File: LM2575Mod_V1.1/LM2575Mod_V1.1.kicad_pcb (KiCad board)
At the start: 2 copper layers, 99.1 x 63.5 mm, 24 parts, among them IC1 LM 2575 T-ADJ, X1 MKDSN1,5_2-5,08, X2 Val**, X3 MKDSN1,5_2-5,08

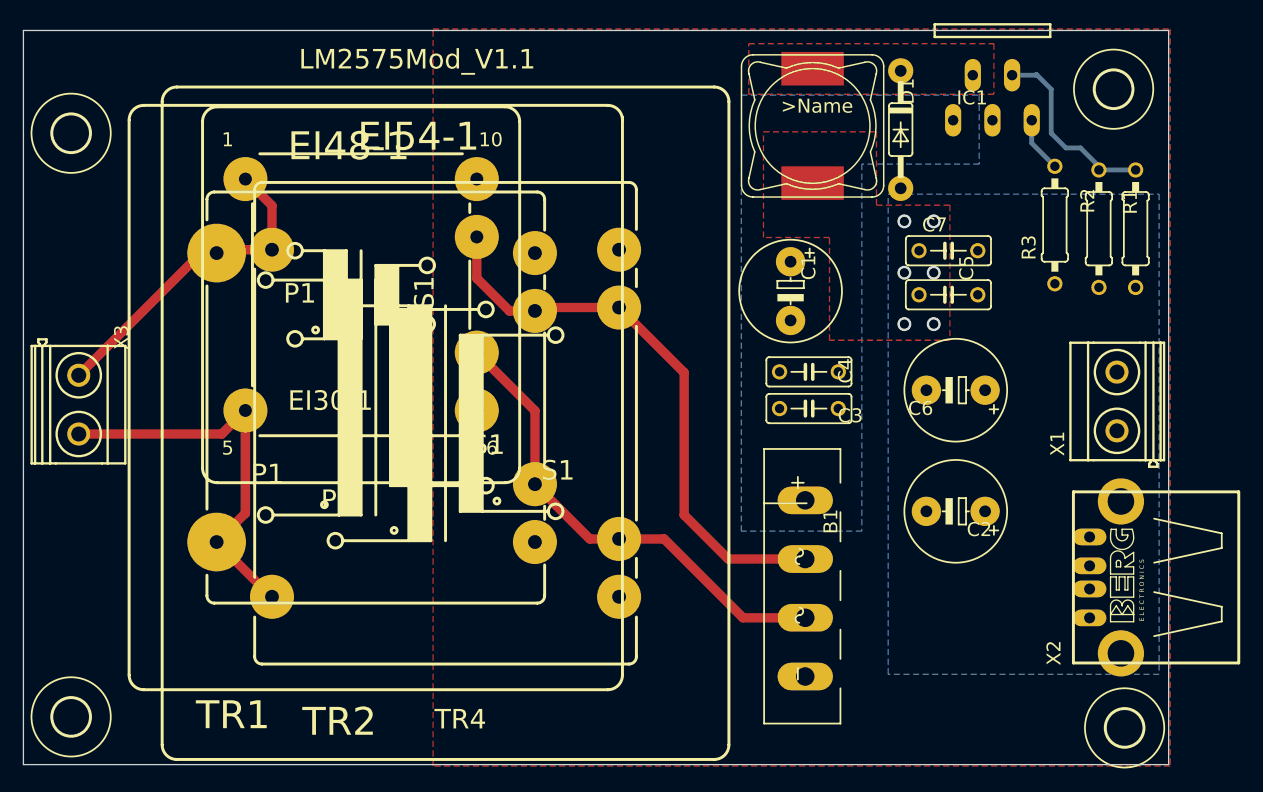
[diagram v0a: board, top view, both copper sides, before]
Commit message: lm2575_pwr V6
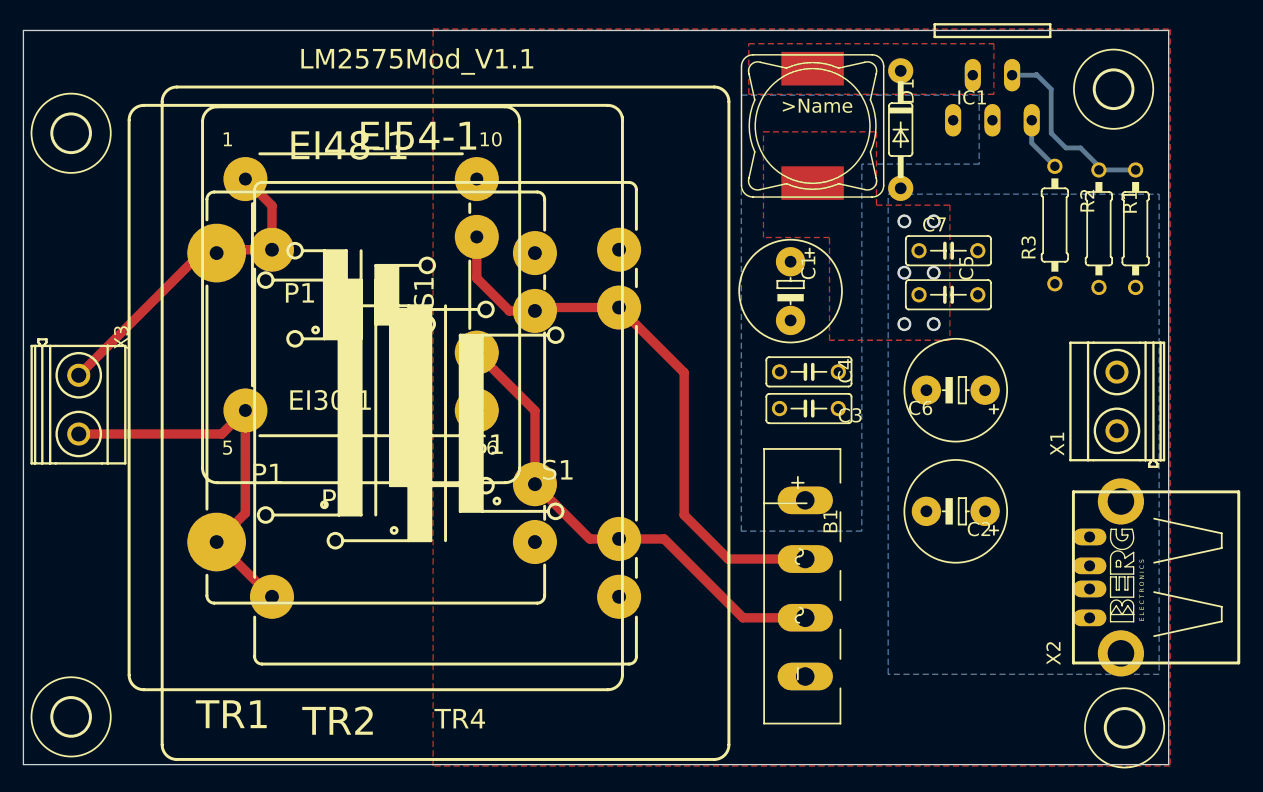
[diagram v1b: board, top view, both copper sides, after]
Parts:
- X2: value Val** -> PN87520
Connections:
- X2 pad 2: Net-(X2-Pad2) -> unconnected-(X2-Pad2)
- X2 pad 3: Net-(X2-Pad3) -> unconnected-(X2-Pad3)
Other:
- net class Default removed
